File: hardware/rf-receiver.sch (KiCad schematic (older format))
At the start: 41 parts, among them J1 InputConP6, J3 Raspberry_Pi_2_3, J8 RF_Shield_One_Piece, P1 ROT_ENC, U1 MIC5504-3.3YM5, U2 CAT24C128, U3 SI5351A-B-GT, Y1 25MHz 20pF

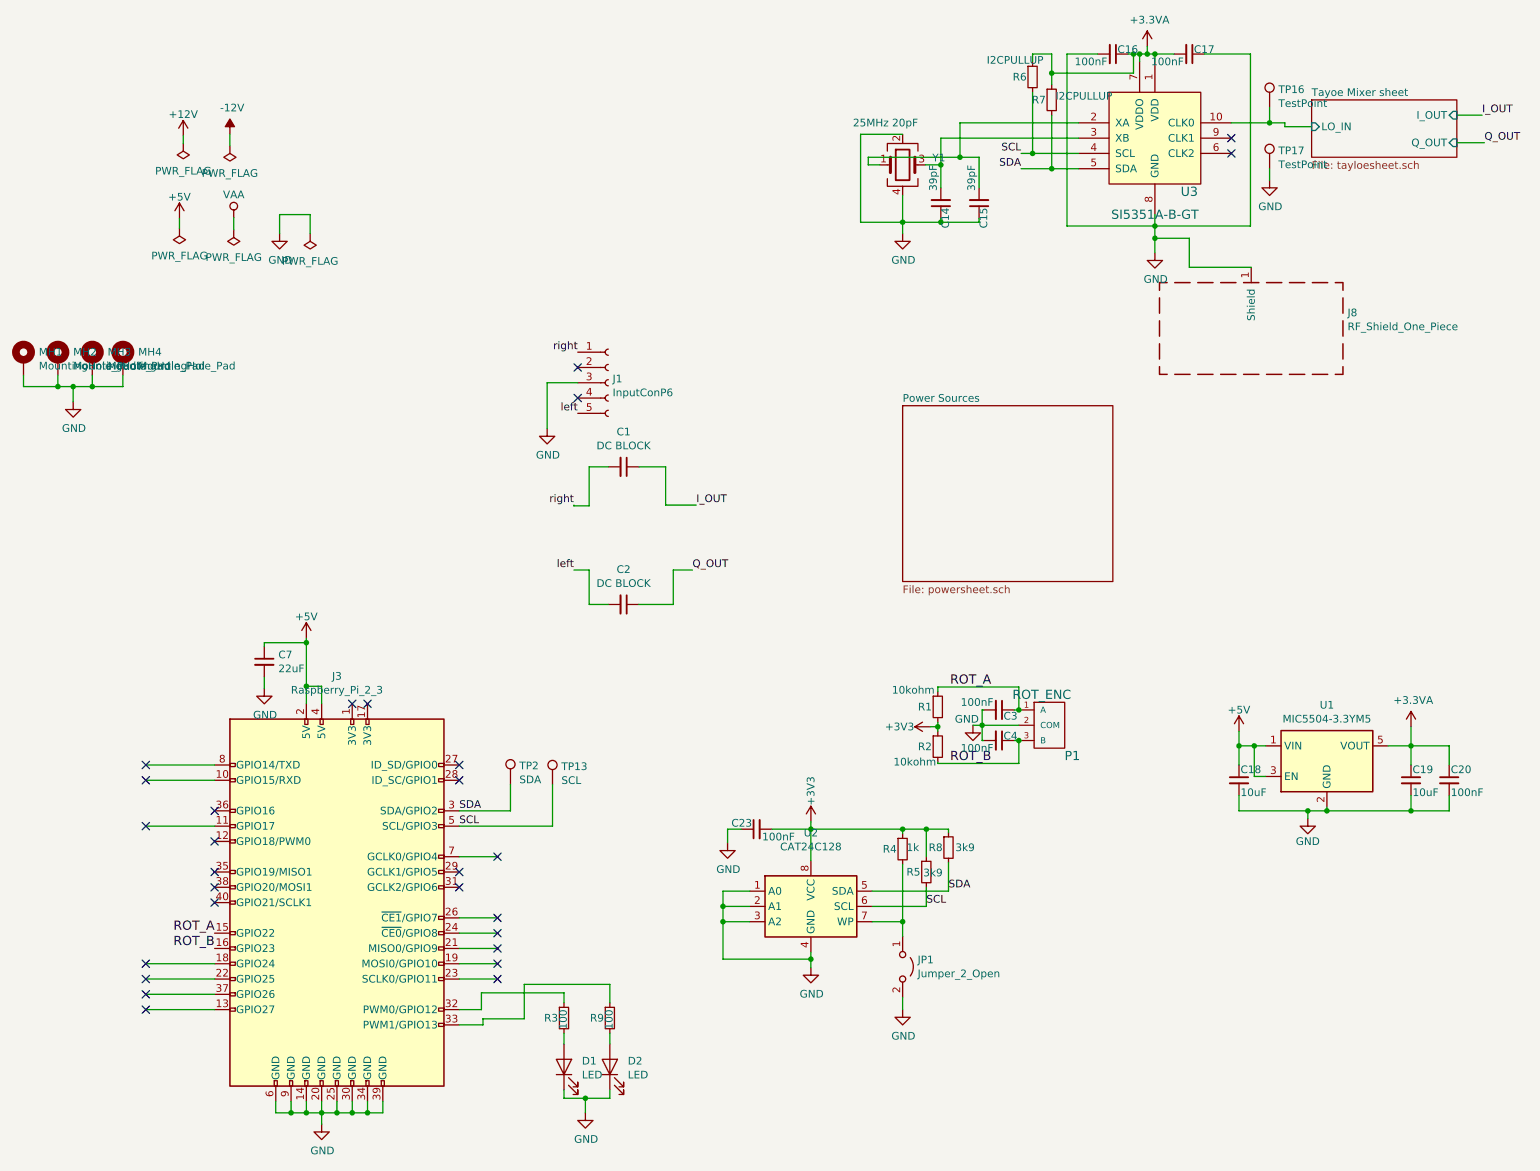
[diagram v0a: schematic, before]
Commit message: Sorry future me
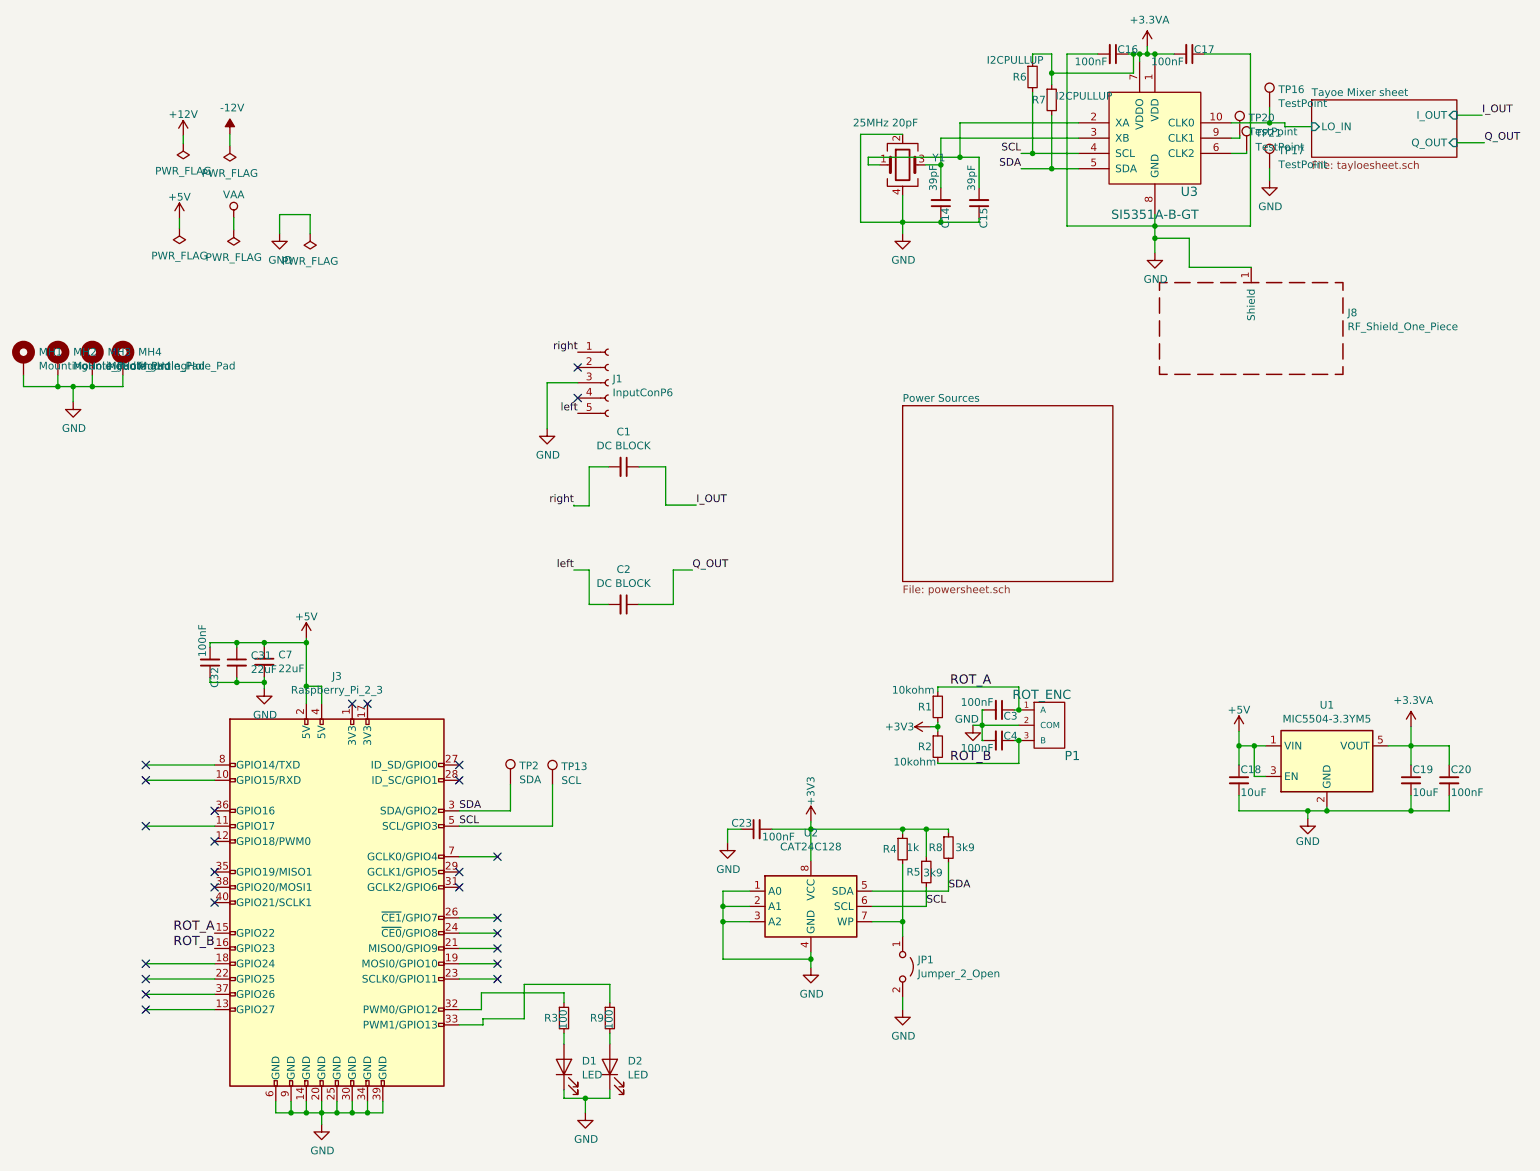
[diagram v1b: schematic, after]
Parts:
- added C31: 22uF, Capacitor_SMD:C_0805_2012Metric, symbol Device:C_Small
- added C32: 100nF, Capacitor_SMD:C_0603_1608Metric, symbol Device:C_Small
- added TP20, TP21: TestPoint, athir:testpoint_probe, symbol Connector:TestPoint
- MH1, MH2, MH3, MH4: footprint MountingHole:MountingHole_2.7mm_M2.5_Pad -> MountingHole:MountingHole_3.2mm_M3_Pad
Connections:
- net +5V: now also C31.1, C32.2
- net GND: now also C31.2, C32.1
- net at U3.6 (CLK2): now also TP21.1
- net at U3.9 (CLK1): now also TP20.1
- no-connect marks 28 -> 26
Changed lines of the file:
@@
 $Descr A4 11693 8268
 encoding utf-8
-Sheet 1 3
+Sheet 1 4
 Title ""
 Date "2019-01-20"
@@
 F 0 "MH1" H 1100 2676 50  0000 L CNN
 F 1 "MountingHole_Pad" H 1100 2585 50  0000 L CNN
-F 2 "MountingHole:MountingHole_2.7mm_M2.5_Pad" H 1000 2625 50  0001 C CNN
+F 2 "MountingHole:MountingHole_3.2mm_M3_Pad" H 1000 2625 50  0001 C CNN
 F 3 "~" H 1000 2625 50  0001 C CNN
 	1    1000 2625
@@
 F 0 "MH2" H 1325 2676 50  0000 L CNN
 F 1 "MountingHole_Pad" H 1325 2585 50  0000 L CNN
-F 2 "MountingHole:MountingHole_2.7mm_M2.5_Pad" H 1225 2625 50  0001 C CNN
+F 2 "MountingHole:MountingHole_3.2mm_M3_Pad" H 1225 2625 50  0001 C CNN
 F 3 "~" H 1225 2625 50  0001 C CNN
 	1    1225 2625
@@
 F 0 "MH3" H 1550 2676 50  0000 L CNN
 F 1 "MountingHole_Pad" H 1550 2585 50  0000 L CNN
-F 2 "MountingHole:MountingHole_2.7mm_M2.5_Pad" H 1450 2625 50  0001 C CNN
+F 2 "MountingHole:MountingHole_3.2mm_M3_Pad" H 1450 2625 50  0001 C CNN
 F 3 "~" H 1450 2625 50  0001 C CNN
 	1    1450 2625
@@
 F 0 "MH4" H 1750 2676 50  0000 L CNN
 F 1 "MountingHole_Pad" H 1750 2585 50  0000 L CNN
-F 2 "MountingHole:MountingHole_2.7mm_M2.5_Pad" H 1650 2625 50  0001 C CNN
+F 2 "MountingHole:MountingHole_3.2mm_M3_Pad" H 1650 2625 50  0001 C CNN
 F 3 "~" H 1650 2625 50  0001 C CNN
 	1    1650 2625
@@
 Wire Wire Line
 	9250 1100 9425 1100
-NoConn ~ 8900 1175
-NoConn ~ 8900 1275
 Text Label 3850 5575 0    50   ~ 0
 SDA
@@
 $EndComp
 Wire Wire Line
-	2575 4775 2575 4700
+	2575 4775 2575 4735
 $Comp
 L power:-12V #PWR?
@@
 Wire Wire Line
 	9150 1450 9150 1375
+$Comp
+L Device:C_Small C?
+U 1 1 5E716223
+P 2395 4605
+AR Path="/5C517D7D/5E716223" Ref="C?"  Part="1"
+AR Path="/5E716223" Ref="C31"  Part="1"
+F 0 "C31" H 2487 4651 50  0000 L CNN
+F 1 "22uF" H 2487 4560 50  0000 L CNN
+F 2 "Capacitor_SMD:C_0805_2012Metric" H 2395 4605 50  0001 C CNN
+F 3 "~" H 2395 4605 50  0001 C CNN
+	1    2395 4605
+	1    0    0    -1
+$EndComp
+Wire Wire Line
+	2575 4475 2395 4475
+Wire Wire Line
+	2395 4475 2395 4505
+Connection ~ 2575 4475
+Wire Wire Line
+	2395 4705 2395 4735
+Wire Wire Line
+	2395 4735 2575 4735
+Connection ~ 2575 4735
+Wire Wire Line
+	2575 4735 2575 4700
+$Comp
+L Device:C_Small C32
+U 1 1 5E733990
+P 2220 4605
+F 0 "C32" V 2190 4635 50  0000 L CNN
+F 1 "100nF" V 2270 4355 50  0000 L CNN
+F 2 "Capacitor_SMD:C_0603_1608Metric" H 2220 4605 50  0001 C CNN
+F 3 "" H 2220 4605 50  0000 C CNN
+	1    2220 4605
+	-1   0    0    1
+$EndComp
+Wire Wire Line
+	2395 4475 2220 4475
+Wire Wire Line
+	2220 4475 2220 4505
+Connection ~ 2395 4475
+Wire Wire Line
+	2220 4705 2220 4735
+Wire Wire Line
+	2220 4735 2395 4735
+Connection ~ 2395 4735
+$Comp
+L Connector:TestPoint TP20
+U 1 1 5E6E2812
+P 8955 1160
+F 0 "TP20" H 9013 1278 50  0000 L CNN
+F 1 "TestPoint" H 9013 1187 50  0000 L CNN
+F 2 "athir:testpoint_probe" H 9155 1160 50  0001 C CNN
+F 3 "~" H 9155 1160 50  0001 C CNN
+	1    8955 1160
+	1    0    0    -1
+$EndComp
+$Comp
+L Connector:TestPoint TP21
+U 1 1 5E6E4E81
+P 9000 1260
+F 0 "TP21" H 9058 1378 50  0000 L CNN
+F 1 "TestPoint" H 9058 1287 50  0000 L CNN
+F 2 "athir:testpoint_probe" H 9200 1260 50  0001 C CNN
+F 3 "~" H 9200 1260 50  0001 C CNN
+	1    9000 1260
+	1    0    0    -1
+$EndComp
+Wire Wire Line
+	8900 1275 9000 1275
+Wire Wire Line
+	9000 1275 9000 1260
+Wire Wire Line
+	8955 1175 8900 1175
+Wire Wire Line
+	8955 1175 8955 1160
 $EndSCHEMATC
